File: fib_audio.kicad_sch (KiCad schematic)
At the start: 1 part, among them U4 WM8960CGEFL

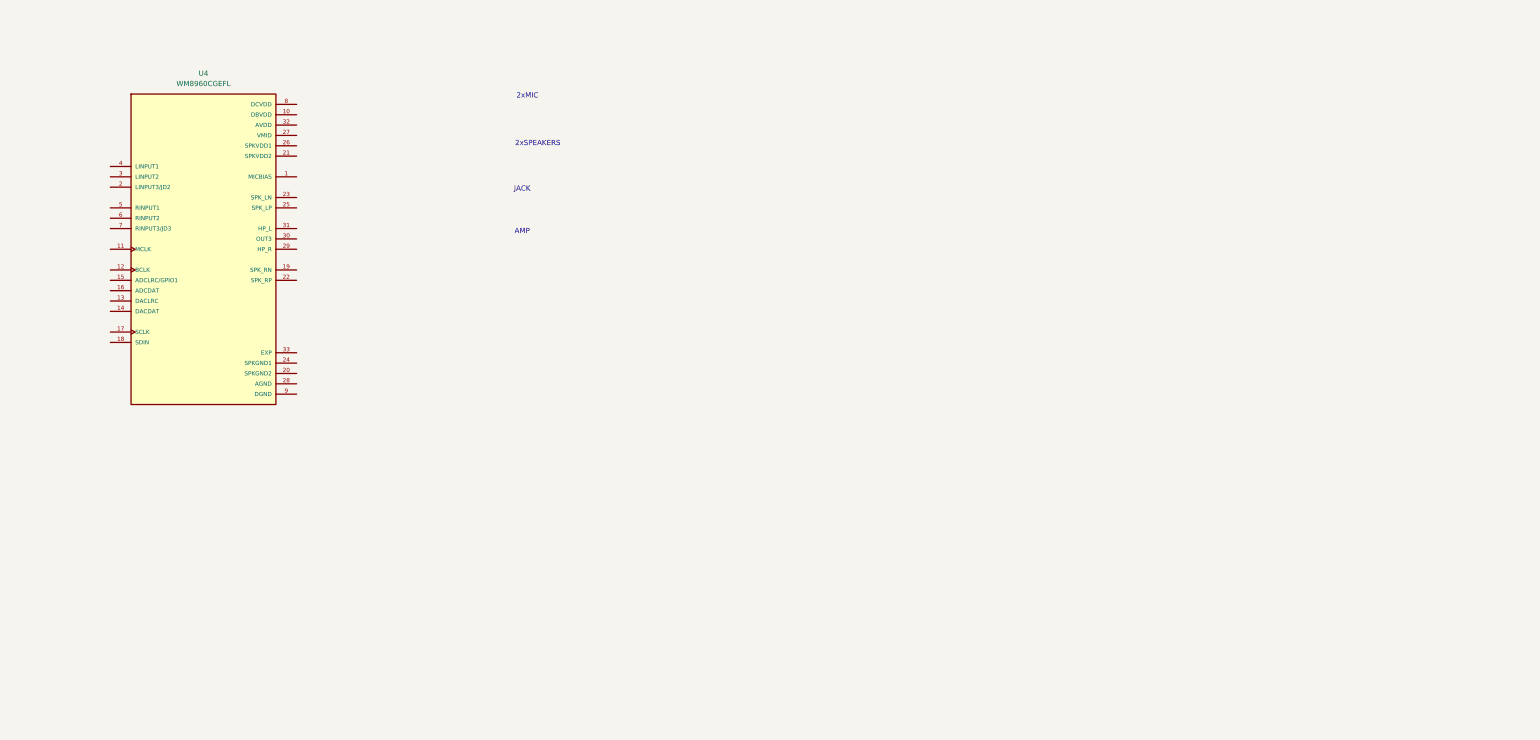
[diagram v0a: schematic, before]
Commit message: added symbol&footprint for orin/sodimm, added a bunch of specs and docs, partially implemented audio, full steam ahead
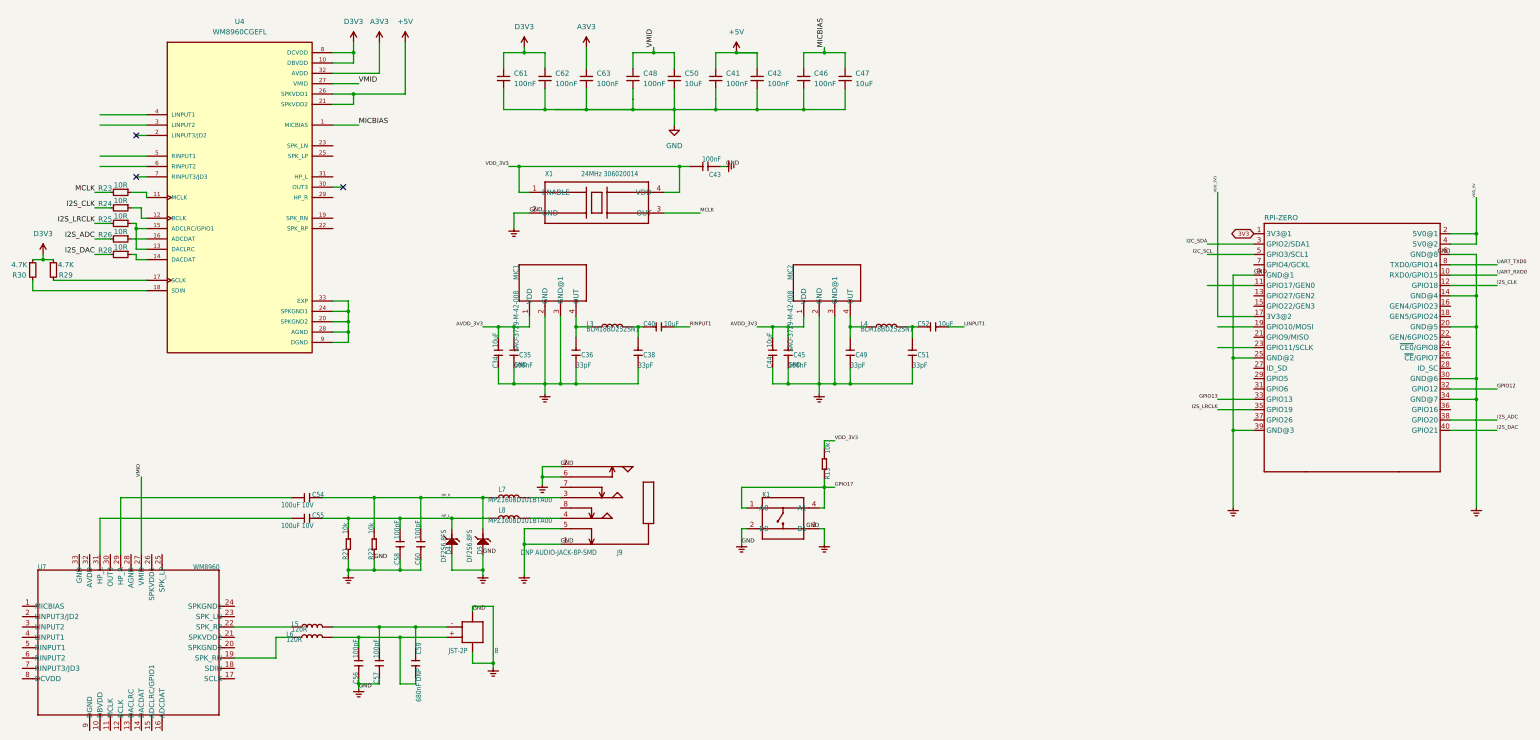
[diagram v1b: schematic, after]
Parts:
- added C34, C40, C44, C52: 10uF, Untitled:C0603, symbol Untitled-eagle-import:CAP-0603
- added C35, C43, C45: 100nF, Untitled:C0402, symbol Untitled-eagle-import:CAP-0402
- added C36, C38, C49, C51: 33pF, Untitled:C0402, symbol Untitled-eagle-import:CAP-0402
- added C41, C42, C46, C48, C61, C62, C63: 100nF, Capacitor_SMD:C_0603_1608Metric, symbol Device:C_Small
- added C47, C50: 10uF, Capacitor_SMD:C_0603_1608Metric, symbol Device:C_Small
- added C54, C55: 100uF 10V, Untitled:C0805, symbol Untitled-eagle-import:CAP-0805
- added C56, C57, C58, C60: 100pF, Untitled:C0402, symbol Untitled-eagle-import:CAP-0402
- added C59: 680nF DNP, Untitled:C0402, symbol Untitled-eagle-import:CAP-0402
- added D4, D5: DF2S6.8FS, Untitled:SOD-923, symbol Untitled-eagle-import:D-ESD-2P'DF2S6.8FS'
- added J8: JST-2P, Untitled:HW2-SMD-2.0-90D, symbol Untitled-eagle-import:JST-2P-SMD'2.0'
- added J9: DNP AUDIO-JACK-8P-SMD, Untitled:AUDIO8P-SMD-3.5-14.5X6.1X4.0MM, symbol Untitled-eagle-import:AUDIO-JACK-8P-SMD'PJ-393'
- added K1: BUTTON-4PDTSM-62K-S-V-T/R(SN431), Untitled:SW4-SMD-6.0X6.0X5.0MM, symbol Untitled-eagle-import:BUTTON-4PDTSM-62K-S-V-T/R(SN431)
- added L3, L4: BLM18BD252SN1, Untitled:L0603, symbol Untitled-eagle-import:INDUCTOR/FERRITE-BEAD'0603'
- added L5, L6: 120R, Untitled:L0603, symbol Untitled-eagle-import:INDUCTOR/FERRITE-BEAD'0603'
- added L7, L8: MPZ1608D101BTA00, Untitled:L0603, symbol Untitled-eagle-import:INDUCTOR/FERRITE-BEAD'0603'
- added MIC1, MIC2: SAO-3729-M-42-008, Untitled:MIC4-SMD-3.76X2.95MM, symbol Untitled-eagle-import:MIC-MSM421A3729H8-C
- added PI1: RPI-ZERO, Untitled:RASPBERRYPI_BASTELSTUBE_V13_RASPI_BOARD_B+_FULL, symbol Untitled-eagle-import:RPI-ZERO
- added R13, R21, R22: 10k, Untitled:R0402, symbol Untitled-eagle-import:Discrete-new_RES-0402
- added R23, R24, R25, R26, R28: 10R, Resistor_SMD:R_0603_1608Metric, symbol Device:R_Small
- added R29, R30: 4.7K, Resistor_SMD:R_0603_1608Metric, symbol Device:R_Small
- added U7: WM8960, Untitled:QFN32G-0.5-5X5MM, symbol Untitled-eagle-import:AMPLIFIER-WM8960
- added X1: 24MHz 306020014, Untitled:OSC4-SMD-2.5X2.0X0.8MM, symbol Untitled-eagle-import:CRYSTAL-OSCILLATOR2.52.0
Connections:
- net MICBIAS: now reaches U4.1 (MICBIAS)
- net MICBIAS: now also C46.1, C47.1
- net D3V3: now reaches U4.10 (DBVDD)
- net D3V3: now also U4.8 (DCVDD), C61.1, C62.1, R29.1, R30.1
- net at U4.11 (MCLK): now also R23.1
- net at U4.12 (BCLK): now also R24.1
- net at U4.13 (DACLRC): now also U4.15 (ADCLRC/GPIO1), R25.1
- net at U4.14 (DACDAT): now also R28.1
- net at U4.16 (ADCDAT): now also R26.1
- net at U4.17 (SCLK): now also R29.2
- net at U4.18 (SDIN): now also R30.2
- net at U4.20 (SPKGND2): now also U4.24 (SPKGND1), U4.28 (AGND), U4.33 (EXP), U4.9 (DGND)
- net +5V: now reaches U4.21 (SPKVDD2)
- net +5V: now also U4.26 (SPKVDD1), C41.1, C42.1
- net VMID: now reaches U4.27 (VMID)
- net VMID: now also C48.1, C50.1, U7.27 (VMID)
- net A3V3: now reaches U4.32 (AVDD)
- net A3V3: now also C63.1
- new net: C51.2, C52.1, L4.2
- new net: C55.1, U7.31 (HP_L)
- new net: C49.2, L4.1, MIC2.4 (OUT)
- new net: J9.3, L7.2
- new net: J9.4, L8.2
- new net: C54.1, U7.29 (HP_R)
- new net: L6.1, U7.19 (SPK_RN)
- new net: C56.2, C59.2, J8.+ (1), L6.2
- new net: C36.2, L3.1, MIC1.4 (OUT)
- new net: L5.1, U7.22 (SPK_RP)
- new net: C57.2, C59.1, J8.- (2), L5.2
- new net: C38.2, C40.1, L3.2
- new net 3V3: PI1.1 (3V3@1)
- new net AVDD_3V3: C34.2, C35.2, C44.2, C45.2, MIC1.1 (VDD), MIC2.1 (VDD)
- new net GND: C34.1, C35.1, C36.1, C38.1, C41.2, C42.2, C43.1, C44.1, C45.1, C46.2, C47.2, C48.2, C49.1, C50.2, C51.1, C56.1, C57.1, C58.1, C60.1, C61.2, C62.2, C63.2, D4.2 (1), D5.2 (1), J8.3, J8.4, J9.1, J9.2, J9.5, J9.6, K1.2 (B0), K1.3 (B1), MIC1.2 (GND), MIC1.3 (GND@1), MIC2.2 (GND), MIC2.3 (GND@1), PI1.14 (GND@4), PI1.20 (GND@5), PI1.25 (GND@2), PI1.30 (GND@6), PI1.34 (GND@7), PI1.39 (GND@3), PI1.6 (GND@8), PI1.9 (GND@1), R21.1, R22.1, X1.2 (GND)
- new net GPIO12: PI1.32 (GPIO12)
- new net GPIO13: PI1.33 (GPIO13)
- new net GPIO17: K1.1 (A0), K1.4 (A1), R13.1
- new net HP_L: C55.2, C58.2, D4.1 (2), L8.1, R21.2
- new net HP_R: C54.2, C60.2, D5.1 (2), L7.1, R22.2
- new net I2C_SCL: PI1.5 (GPIO3/SCL1)
- new net I2C_SDA: PI1.3 (GPIO2/SDA1)
- new net I2S_ADC: PI1.38 (GPIO20), R26.2
- new net I2S_CLK: PI1.12 (GPIO18), R24.2
- new net I2S_DAC: PI1.40 (GPIO21), R28.2
- new net I2S_LRCLK: PI1.35 (GPIO19), R25.2
- new net LINPUT1: C52.2
- new net MCLK: R23.2, X1.3 (OUT)
- new net RINPUT1: C40.2
- new net UART_RXD0: PI1.10 (RXD0/GPIO15)
- new net UART_TXD0: PI1.8 (TXD0/GPIO14)
- new net VDD_3V3: C43.2, PI1.17 (3V3@2), R13.2, X1.1 (ENABLE), X1.4 (VDD)
- new net VDD_5V: PI1.2 (5V0@1), PI1.4 (5V0@2)
- no-connect marks 0 -> 3
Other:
- note removed: "2xMIC"
- note removed: "2xSPEAKERS"
- note removed: "AMP"
- note removed: "JACK"
- moved on the sheet: U4
